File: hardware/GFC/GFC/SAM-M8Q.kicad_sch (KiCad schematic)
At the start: 5 parts, among them U4 SAM-M8Q

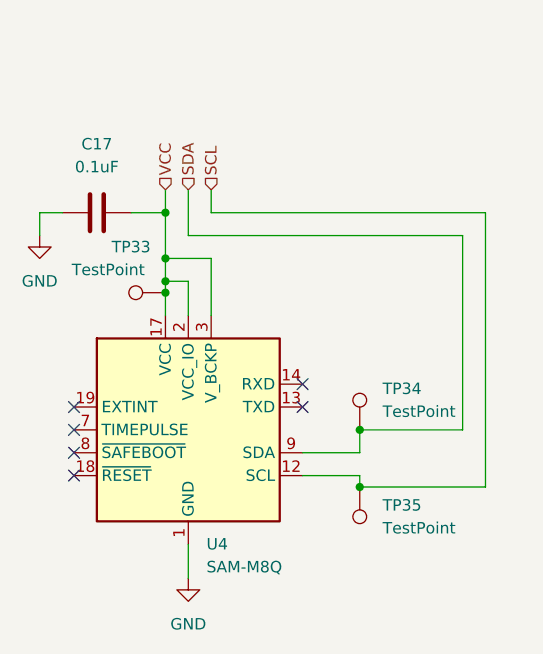
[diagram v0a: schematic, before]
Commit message: sync
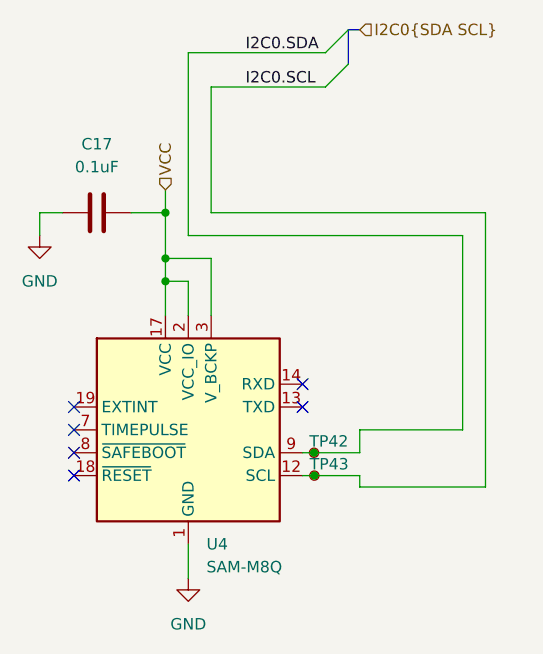
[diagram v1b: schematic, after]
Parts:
- removed TP33, TP34, TP35: TestPoint, TestPoint:TestPoint_Pad_D1.0mm, symbol Connector:TestPoint
- added TP42, TP43: Test Point, TestPoint:TestPoint_Pad_D1.0mm, symbol Connector:TestPoint_Small
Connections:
- net SCL renamed I2C0.SCL
- net I2C0.SCL: now also TP43.1
- net SDA renamed I2C0.SDA
- net I2C0.SDA: now also TP42.1
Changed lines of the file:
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@@
   (junction (at 130.81 63.5) (diameter 0) (color 0 0 0 0)
+  )
+  (junction (at 147.3561 92.71) (diameter 0) (color 0 0 0 0)
   )
   (junction (at 130.81 68.58) (diameter 0) (color 0 0 0 0)
   )
-  (junction (at 152.4 87.63) (diameter 0) (color 0 0 0 0)
+  (junction (at 147.32 90.17) (diameter 0) (color 0 0 0 0)
   )
   (junction (at 130.81 71.12) (diameter 0) (color 0 0 0 0)
-  )
-  (junction (at 130.81 72.39) (diameter 0) (color 0 0 0 0)
-  )
-  (junction (at 152.4 93.98) (diameter 0) (color 0 0 0 0)
   )
   (no_connect (at 120.65 92.71))
@@
   (no_connect (at 146.05 85.09))
   (no_connect (at 120.65 85.09))
+  (bus_entry (at 151.13 43.18) (size -2.54 2.54)
+    (stroke (width 0) (type default) (color 0 0 0 0))
+  )
+  (bus_entry (at 151.13 46.99) (size -2.54 2.54)
+    (stroke (width 0) (type default) (color 0 0 0 0))
+  )
   (wire (pts (xy 152.4 93.98) (xy 166.37 93.98))
     (stroke (width 0) (type default) (color 0 0 0 0))
   )
-  (wire (pts (xy 133.35 66.04) (xy 133.35 60.96))
+  (wire (pts (xy 146.05 90.17) (xy 147.32 90.17))
     (stroke (width 0) (type default) (color 0 0 0 0))
   )
-  (wire (pts (xy 146.05 90.17) (xy 152.4 90.17))
+  (bus (pts (xy 152.4 43.18) (xy 151.13 43.18))
     (stroke (width 0) (type default) (color 0 0 0 0))
   )
-  (wire (pts (xy 130.81 71.12) (xy 130.81 72.39))
+  (wire (pts (xy 130.81 71.12) (xy 130.81 74.93))
     (stroke (width 0) (type default) (color 0 0 0 0))
   )
@@
   )
   (wire (pts (xy 166.37 63.5) (xy 135.89 63.5))
+    (stroke (width 0) (type default) (color 0 0 0 0))
+  )
+  (wire (pts (xy 148.59 45.72) (xy 133.35 45.72))
     (stroke (width 0) (type default) (color 0 0 0 0))
   )
@@
     (stroke (width 0) (type default) (color 0 0 0 0))
   )
-  (wire (pts (xy 130.81 72.39) (xy 130.81 74.93))
-    (stroke (width 0) (type default) (color 0 0 0 0))
-  )
   (wire (pts (xy 130.81 68.58) (xy 130.81 71.12))
     (stroke (width 0) (type default) (color 0 0 0 0))
@@
     (stroke (width 0) (type default) (color 0 0 0 0))
   )
-  (wire (pts (xy 146.05 92.71) (xy 152.4 92.71))
+  (wire (pts (xy 146.05 92.71) (xy 147.3561 92.71))
+    (stroke (width 0) (type default) (color 0 0 0 0))
+  )
+  (wire (pts (xy 147.32 90.17) (xy 152.4 90.17))
     (stroke (width 0) (type default) (color 0 0 0 0))
   )
   (wire (pts (xy 130.81 60.96) (xy 130.81 63.5))
+    (stroke (width 0) (type default) (color 0 0 0 0))
+  )
+  (bus (pts (xy 151.13 43.18) (xy 151.13 46.99))
+    (stroke (width 0) (type default) (color 0 0 0 0))
+  )
+  (wire (pts (xy 147.3561 92.71) (xy 152.4 92.71))
     (stroke (width 0) (type default) (color 0 0 0 0))
   )
@@
   )
   (wire (pts (xy 130.81 63.5) (xy 130.81 68.58))
+    (stroke (width 0) (type default) (color 0 0 0 0))
+  )
+  (wire (pts (xy 135.89 49.53) (xy 148.59 49.53))
     (stroke (width 0) (type default) (color 0 0 0 0))
   )
@@
     (stroke (width 0) (type default) (color 0 0 0 0))
   )
-  (wire (pts (xy 135.89 63.5) (xy 135.89 60.96))
+  (wire (pts (xy 135.89 49.53) (xy 135.89 63.5))
     (stroke (width 0) (type default) (color 0 0 0 0))
   )
@@
     (stroke (width 0) (type default) (color 0 0 0 0))
   )
-  (hierarchical_label "SCL" (shape input) (at 135.89 60.96 90)
-    (effects (font (size 1.27 1.27)) (justify left))
+  (wire (pts (xy 133.35 45.72) (xy 133.35 66.04))
+    (stroke (width 0) (type default) (color 0 0 0 0))
   )
-  (hierarchical_label "SDA" (shape input) (at 133.35 60.96 90)
+  (label "I2C0.SDA" (at 139.7 45.72 0)
+    (effects (font (size 1.27 1.27)) (justify left bottom))
+  )
+  (label "I2C0.SCL" (at 139.7 49.53 0)
+    (effects (font (size 1.27 1.27)) (justify left bottom))
+  )
+  (hierarchical_label "I2C0{SDA SCL}" (shape input) (at 152.4 43.18 0)
     (effects (font (size 1.27 1.27)) (justify left))
   )
@@
     (effects (font (size 1.27 1.27)) (justify left))
   )
-  (symbol (lib_id "Connector:TestPoint") (at 152.4 87.63 0) (unit 1)
-    (in_bom yes) (on_board yes) (fields_autoplaced)
-    (property "Reference" "TP34" (id 0) (at 154.94 83.0579 0)
+  (symbol (lib_id "Connector:TestPoint_Small") (at 147.3561 92.71 0) (mirror y) (unit 1)
+    (in_bom yes) (on_board yes)
+    (property "Reference" "TP43" (id 0) (at 151.1661 91.44 0)
       (effects (font (size 1.27 1.27)) (justify left))
     )
-    (property "Value" "TestPoint" (id 1) (at 154.94 85.5979 0)
-      (effects (font (size 1.27 1.27)) (justify left))
+    (property "Value" "Test Point" (id 1) (at 146.0861 93.9799 0)
+      (effects (font (size 1.27 1.27)) (justify left) hide)
     )
-    (property "Footprint" "TestPoint:TestPoint_Pad_D1.0mm" (id 2) (at 157.48 87.63 0)
+    (property "Footprint" "TestPoint:TestPoint_Pad_D1.0mm" (id 2) (at 142.2761 92.71 0)
       (effects (font (size 1.27 1.27)) hide)
     )
-    (property "Datasheet" "~" (id 3) (at 157.48 87.63 0)
+    (property "Datasheet" "~" (id 3) (at 142.2761 92.71 0)
       (effects (font (size 1.27 1.27)) hide)
     )
@@
     (pin "2")
   )
-  (symbol (lib_id "Connector:TestPoint") (at 130.81 72.39 90) (unit 1)
+  (symbol (lib_id "Connector:TestPoint_Small") (at 147.32 90.17 0) (mirror y) (unit 1)
     (in_bom yes) (on_board yes)
-    (property "Reference" "TP33" (id 0) (at 127 67.31 90))
-    (property "Value" "TestPoint" (id 1) (at 124.46 69.85 90))
-    (property "Footprint" "TestPoint:TestPoint_Pad_D1.0mm" (id 2) (at 130.81 67.31 0)
+    (property "Reference" "TP42" (id 0) (at 151.13 88.9 0)
+      (effects (font (size 1.27 1.27)) (justify left))
+    )
+    (property "Value" "Test Point" (id 1) (at 146.05 91.4399 0)
+      (effects (font (size 1.27 1.27)) (justify left) hide)
+    )
+    (property "Footprint" "TestPoint:TestPoint_Pad_D1.0mm" (id 2) (at 142.24 90.17 0)
       (effects (font (size 1.27 1.27)) hide)
     )
-    (property "Datasheet" "~" (id 3) (at 130.81 67.31 0)
+    (property "Datasheet" "~" (id 3) (at 142.24 90.17 0)
       (effects (font (size 1.27 1.27)) hide)
     )
@@
       (effects (font (size 1.27 1.27)) hide)
     )
-    (pin "1")
-  )
-  (symbol (lib_id "Connector:TestPoint") (at 152.4 93.98 180) (unit 1)
-    (in_bom yes) (on_board yes) (fields_autoplaced)
-    (property "Reference" "TP35" (id 0) (at 154.94 96.0119 0)
-      (effects (font (size 1.27 1.27)) (justify right))
-    )
-    (property "Value" "TestPoint" (id 1) (at 154.94 98.5519 0)
-      (effects (font (size 1.27 1.27)) (justify right))
-    )
-    (property "Footprint" "TestPoint:TestPoint_Pad_D1.0mm" (id 2) (at 147.32 93.98 0)
-      (effects (font (size 1.27 1.27)) hide)
-    )
-    (property "Datasheet" "~" (id 3) (at 147.32 93.98 0)
-      (effects (font (size 1.27 1.27)) hide)
-    )
